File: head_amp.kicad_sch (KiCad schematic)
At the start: 24 parts, among them J1 Conn_01x15, J2 Conn_01x15, J3 Conn_01x05, J4 Conn_01x03, J5 Left_Speaker, J6 Left_Speaker, J7 Left_Speaker, J8 Left_Speaker, M1 Fan, Q1 AO3401A, Q2 AO3400A, U2 Headphone Jack

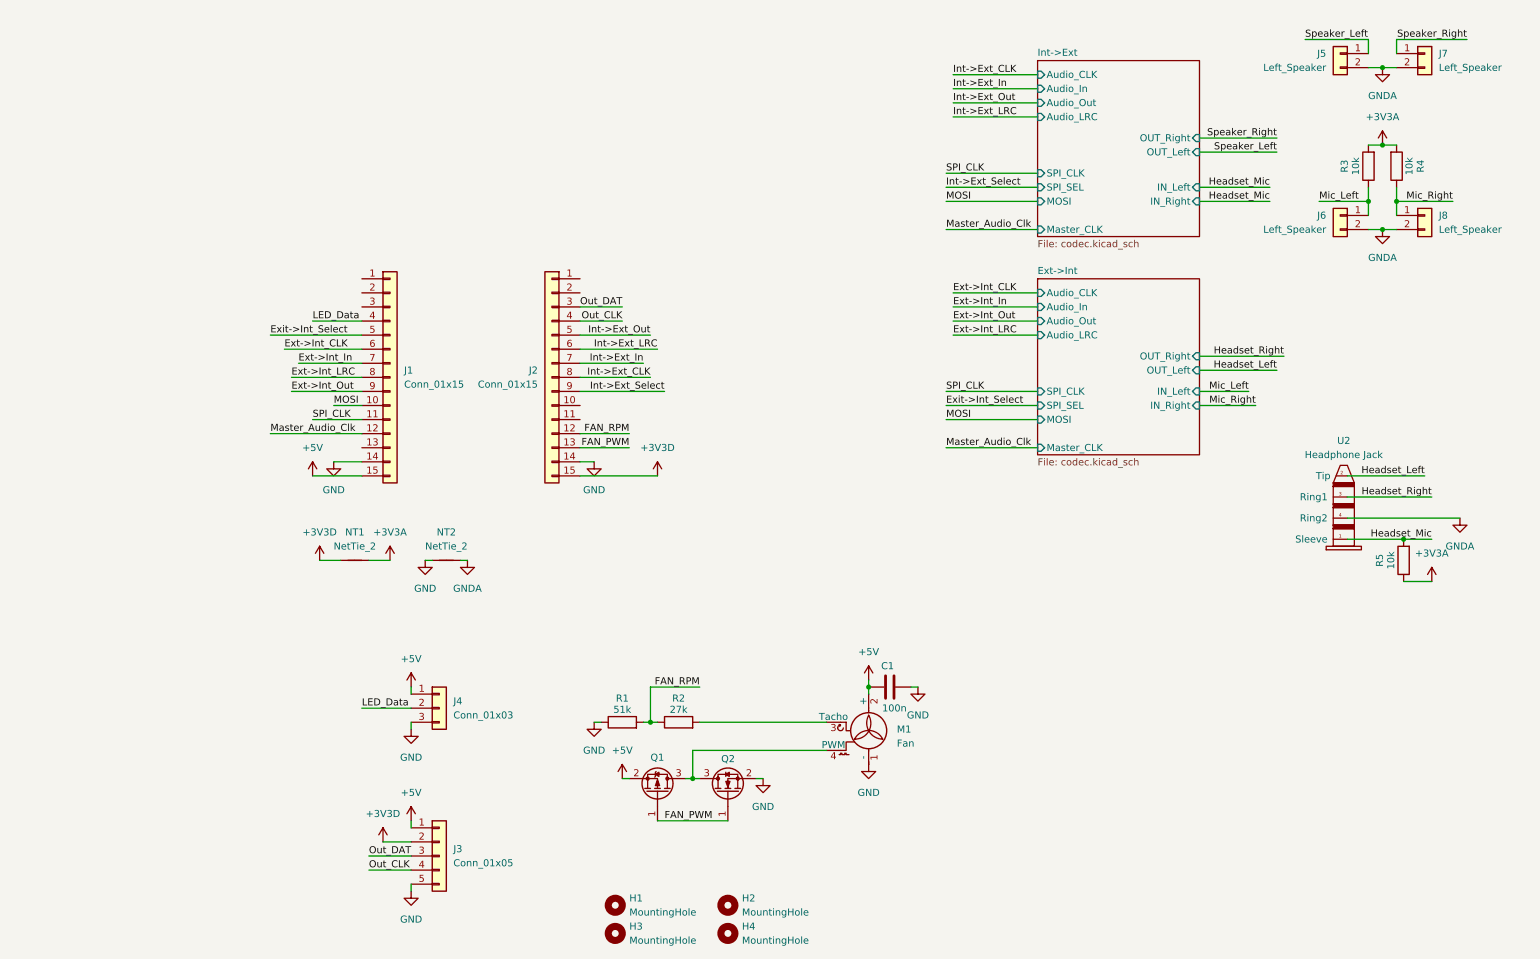
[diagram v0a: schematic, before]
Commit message: feat: overhaul
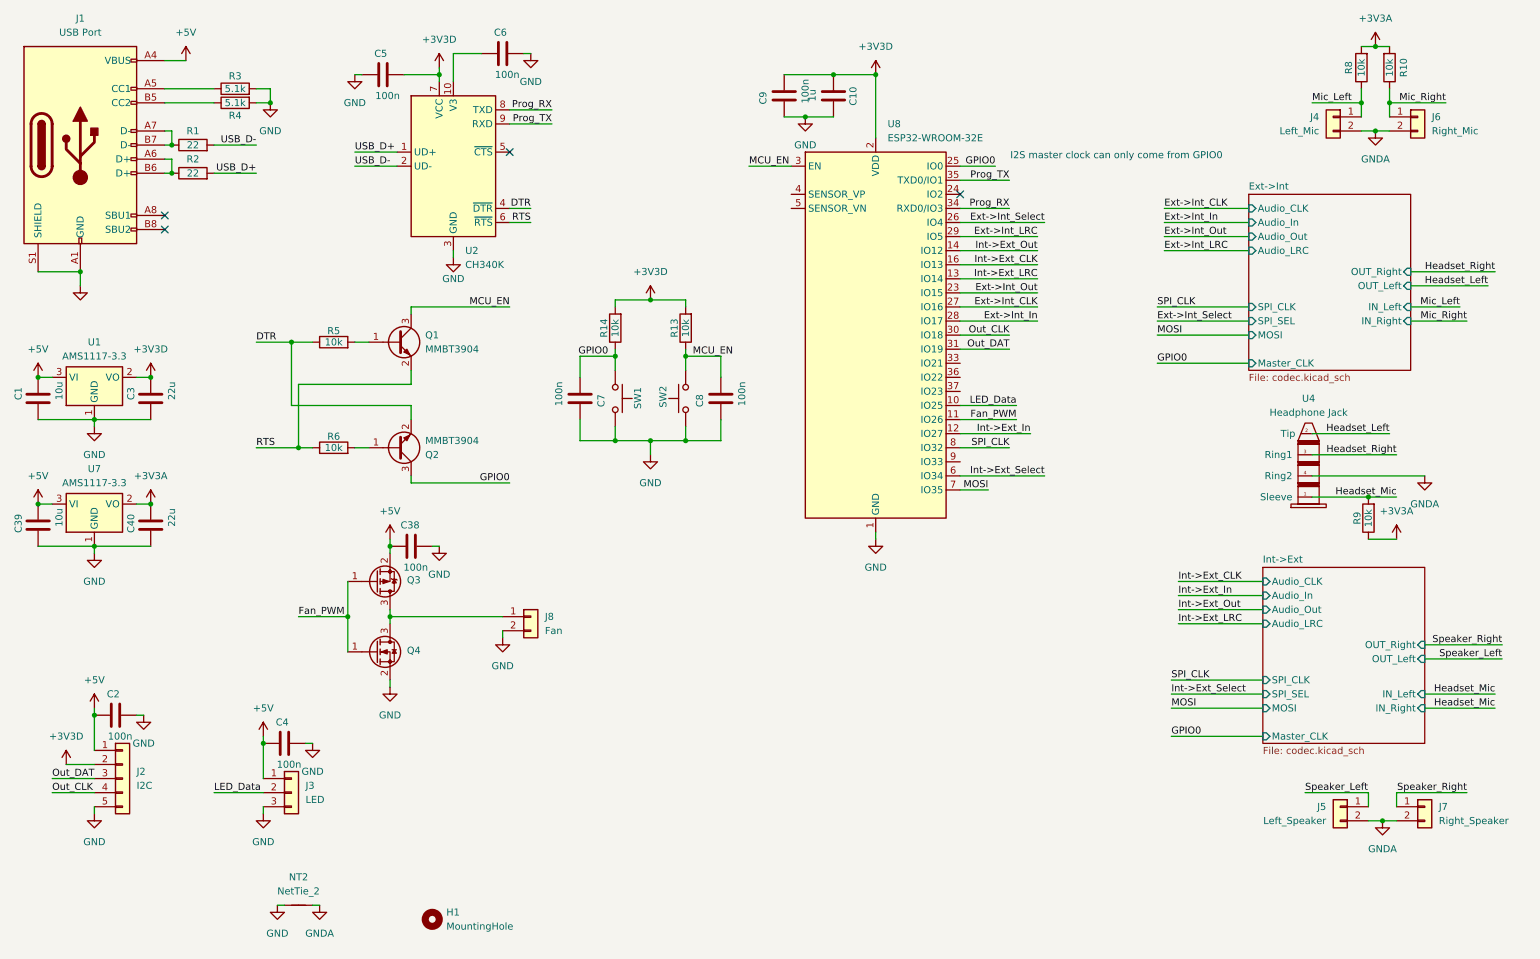
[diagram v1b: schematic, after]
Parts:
- removed H2, H3, H4: MountingHole, MountingHole:MountingHole_2.2mm_M2, symbol Mechanical:MountingHole
- removed J1, J2: Conn_01x15, Connector_PinHeader_2.54mm:PinHeader_1x15_P2.54mm_Vertical, symbol Connector_Generic:Conn_01x15
- removed M1: Fan, A2543WR-4P:MOLEX_22053041, symbol Motor:Fan_Tacho_PWM
- removed NT1: NetTie_2, NetTie:NetTie-2_THT_Pad1.0mm, symbol Device:NetTie_2
- removed Q1: AO3401A, Package_TO_SOT_SMD:SOT-23, symbol Transistor_FET:AO3401A
- removed Q2: AO3400A, Package_TO_SOT_SMD:SOT-23, symbol Transistor_FET:AO3400A
- added C10: 1u, Capacitor_SMD:C_0603_1608Metric, symbol Device:C
- added C2, C38, C4, C9: 100n, Capacitor_SMD:C_0603_1608Metric, symbol Device:C
- added C3, C40: 22u, Capacitor_SMD:C_0603_1608Metric, symbol Device:C
- added C39: 10u, Capacitor_SMD:C_0603_1608Metric, symbol Device:C
- added C5, C6, C7, C8: 100n, Capacitor_SMD:C_0402_1005Metric, symbol Device:C
- added J1: USB Port, Connector_USB:USB_C_Receptacle_GCT_USB4105-xx-A_16P_TopMnt_Horizontal, symbol Connector:USB_C_Receptacle_USB2.0_16P
- added J8: Fan, Connector_JST:JST_EH_S2B-EH_1x02_P2.50mm_Horizontal, symbol Connector_Generic:Conn_01x02
- added Q1, Q2: MMBT3904, Package_TO_SOT_SMD:SOT-23, symbol Transistor_BJT:MMBT3904
- added Q3: AO3401A, Package_TO_SOT_SMD:SOT-23, symbol Transistor_FET:AO3401A
- added Q4: AO3400A, Package_TO_SOT_SMD:SOT-23, symbol Transistor_FET:AO3400A
- added R13, R14, R5, R6: 10k, Resistor_SMD:R_0402_1005Metric, symbol Device:R
- added R3, R4: 5.1k, Resistor_SMD:R_0402_1005Metric, symbol Device:R
- added SW1, SW2: SW_Push, Button_Switch_SMD:SW_SPST_TS-1088-xR020, symbol Switch:SW_Push
- added U1, U7: AMS1117-3.3, Package_TO_SOT_SMD:SOT-223-3_TabPin2, symbol Regulator_Linear:AMS1117-3.3
- added U2: CH340K, Package_SO:SSOP-10-1EP_3.9x4.9mm_P1mm_EP2.1x3.3mm, symbol Interface_USB:CH340K
- added U8: ESP32-WROOM-32E, RF_Module:ESP32-WROOM-32E, symbol RF_Module:ESP32-WROOM-32E
- C1: value 100n -> 10u; LCSC (none) -> C19702
- H1: footprint MountingHole:MountingHole_2.2mm_M2 -> MountingHole:MountingHole_3.2mm_M3
- J2: renamed from J3; value Conn_01x05 -> I2C
- J3: renamed from J4; value Conn_01x03 -> LED
- J4: renamed from J6; value Left_Speaker -> Left_Mic
- J6: renamed from J8; value Left_Speaker -> Right_Mic
- J7: value Left_Speaker -> Right_Speaker
- NT2: footprint NetTie:NetTie-2_THT_Pad1.0mm -> NetTie:NetTie-2_SMD_Pad2.0mm
- R1: value 51k -> 22; footprint Resistor_SMD:R_0603_1608Metric -> Resistor_SMD:R_0402_1005Metric; LCSC (none) -> C25092
- R10: renamed from R4; footprint Resistor_SMD:R_0603_1608Metric -> Resistor_SMD:R_0402_1005Metric; LCSC (none) -> C25744
- R2: value 27k -> 22; footprint Resistor_SMD:R_0603_1608Metric -> Resistor_SMD:R_0402_1005Metric; LCSC (none) -> C25092
- R8: renamed from R3; footprint Resistor_SMD:R_0603_1608Metric -> Resistor_SMD:R_0402_1005Metric; LCSC (none) -> C25744
- R9: renamed from R5; footprint Resistor_SMD:R_0603_1608Metric -> Resistor_SMD:R_0402_1005Metric; LCSC (none) -> C25744
- renumbered U2 to U4
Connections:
- net +3V3A: now also C40.2, U7.2 (VO)
- net +3V3D: now also C10.1, C3.2, C5.2, C9.2, R13.2, R14.2, U1.2 (VO), U2.7 (VCC), U8.2 (VDD)
- net +5V: now also C1.2, C2.1, C38.1, C39.2, C4.1, J1.A4 (VBUS), J1.A9 (VBUS), J1.B4 (VBUS), J1.B9 (VBUS), Q3.2 (S), U1.3 (VI), U7.3 (VI); no longer C1.1
- net Ext->Int_CLK: now also U8.27 (IO16)
- net Ext->Int_In: now also U8.28 (IO17)
- net Ext->Int_LRC: now also U8.29 (IO5)
- net Ext->Int_Out: now also U8.23 (IO15)
- net GND: now also C1.1, C10.2, C2.2, C3.1, C38.2, C39.1, C4.2, C40.1, C5.1, C6.2, C7.1, C8.1, C9.1, J1.A1 (GND), J1.A12 (GND), J1.B1 (GND), J1.B12 (GND), J1.S1 (SHIELD), J8.2 (Pin_2), Q4.2 (S), R3.2, R4.2, SW1.1, SW2.1, U1.1 (GND), U2.11 (GND), U2.3 (GND), U7.1 (GND), U8.1 (GND), U8.15 (GND), U8.38 (GND), U8.39 (GND); no longer C1.2, R1.1
- net Int->Ext_CLK: now also U8.16 (IO13)
- net Int->Ext_In: now also U8.12 (IO27)
- net Int->Ext_LRC: now also U8.13 (IO14)
- net Int->Ext_Out: now also U8.14 (IO12)
- net Int->Ext_Select: now also U8.6 (IO34)
- net LED_Data: now also U8.10 (IO25)
- net MOSI: now also U8.7 (IO35)
- net Out_CLK: now also U8.30 (IO18)
- net Out_DAT: now also U8.31 (IO19)
- net SPI_CLK: now also U8.8 (IO32)
- net USB_D+: now reaches R2.2
- net USB_D+: now also U2.1 (UD+)
- net FAN_RPM: no longer names the net of R2.1
- net FAN_RPM: now also J1.A6 (D+), J1.B6 (D+); no longer R1.2
- new net: J8.1 (Pin_1), Q3.3 (D), Q4.3 (D)
- new net: J1.A7 (D-), J1.B7 (D-), R1.1
- new net: Q2.1 (B), R6.2
- new net: J1.B5 (CC2), R4.1
- new net: Q1.1 (B), R5.2
- new net: J1.A5 (CC1), R3.1
- new net: C6.1, U2.10 (V3)
- new net DTR: Q2.2 (E), R5.1, U2.4 (~{DTR})
- new net Ext->Int_Select: U8.26 (IO4)
- new net Fan_PWM: Q3.1 (G), Q4.1 (G), U8.11 (IO26)
- new net GPIO0: C7.2, Q2.3 (C), R14.1, SW1.2, U8.25 (IO0)
- new net MCU_EN: C8.2, Q1.3 (C), R13.1, SW2.2, U8.3 (EN)
- new net Prog_RX: U2.8 (TXD), U8.34 (RXD0/IO3)
- new net Prog_TX: U2.9 (RXD), U8.35 (TXD0/IO1)
- new net RTS: Q1.2 (E), R6.1, U2.6 (~{RTS})
- new net USB_D-: R1.2, U2.2 (UD-)
- no-connect marks 0 -> 4
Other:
- note added: "I2S master clock can only come from GPIO0"
- moved on the sheet: H1, J2, J3, J4, J5, J6, J7, NT2, R10, R8, R9, U4
